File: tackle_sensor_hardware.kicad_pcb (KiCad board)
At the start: 4 copper layers, 47 x 59.7 mm, 72 parts, among them J1 Conn_ARM_JTAG_SWD_10, J2 Conn_01x02_Male, J3 Conn_01x03_Male, J4 Conn_01x04_Male, Q1 DMP4051LK3, Q2 NCE0110K, SW1 PTS645SL43SMTR92 LFS, SW2 SW_DPDT_x2, T1 DRQ125-330-R, U1 STM32G031Fx, U2 LM3488, U3 LIS2DE12, U4 LD1117S33TR_SOT223, U5 ULN2003ADR

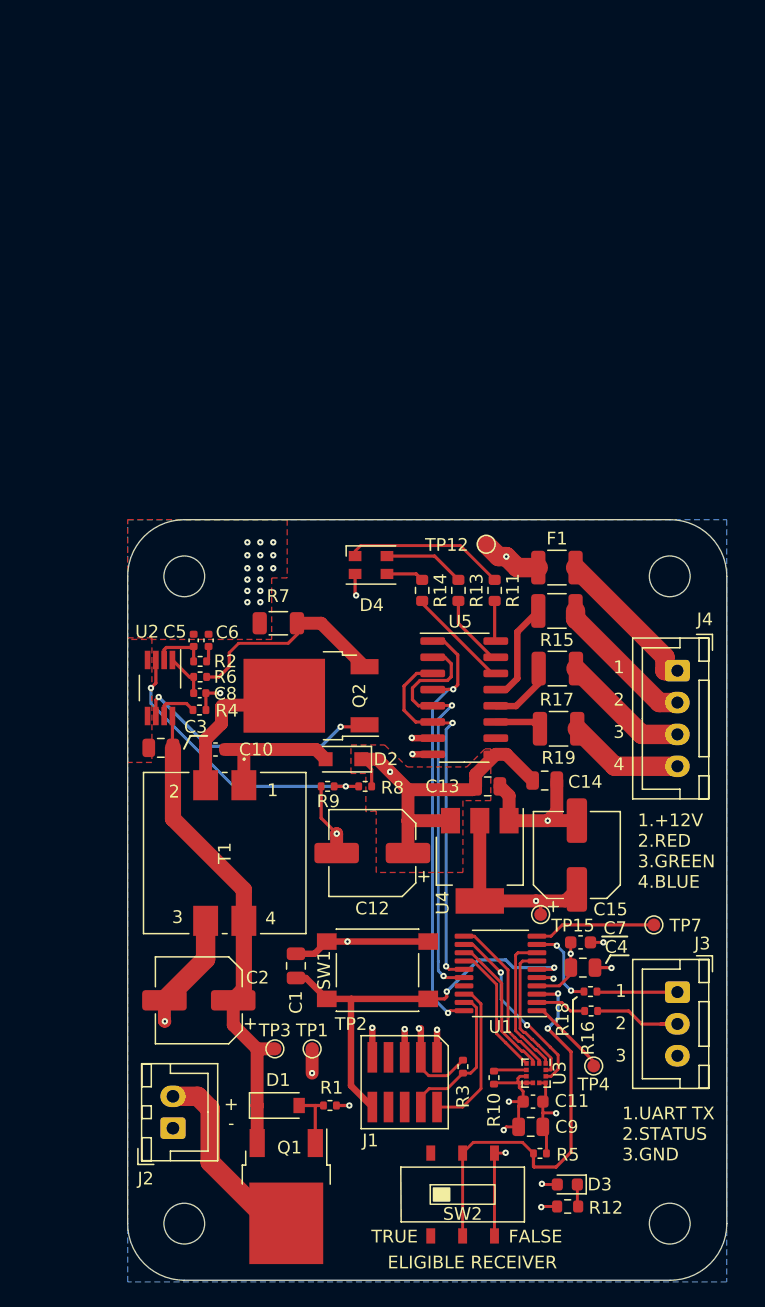
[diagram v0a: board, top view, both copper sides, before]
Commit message: - add reference PDFs and dimensions to the layout
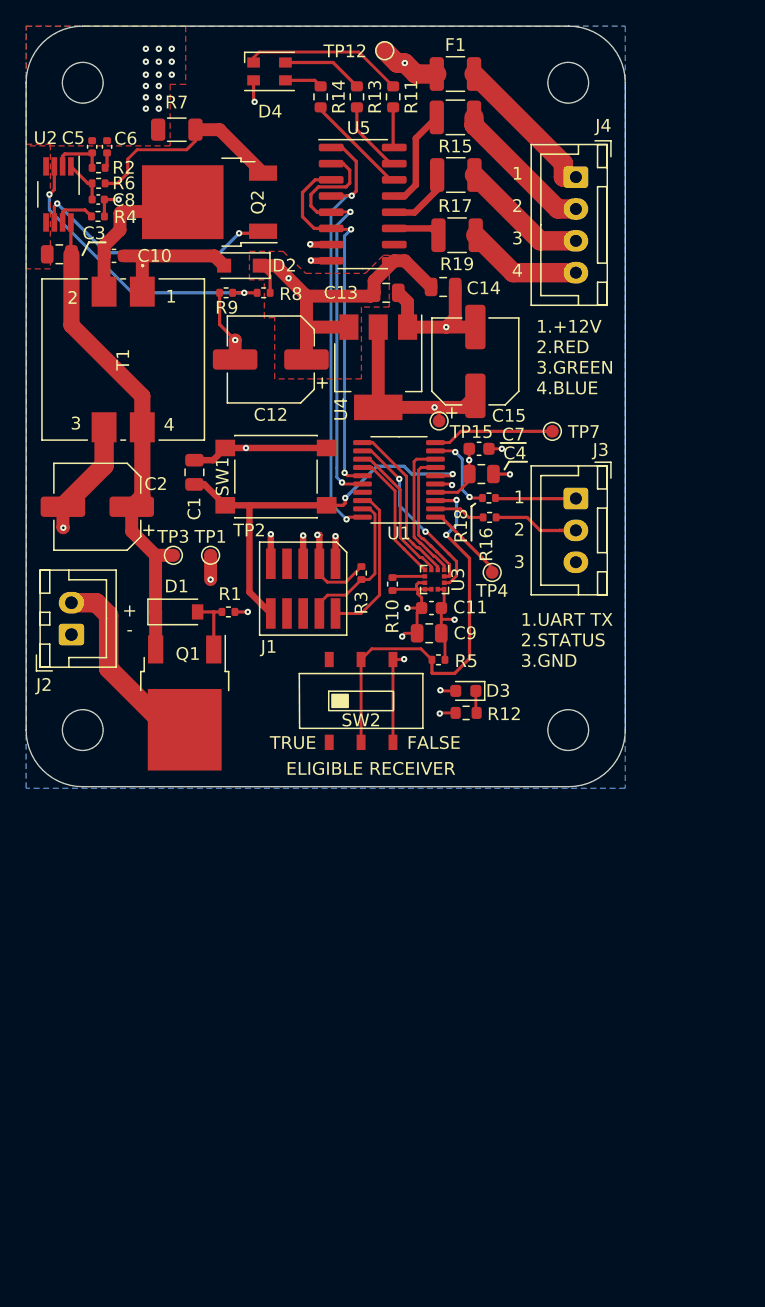
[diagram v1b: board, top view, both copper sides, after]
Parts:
- moved C14 39.5 mm to (145.4, 51.6)
- moved C15 39.5 mm to (147.9, 57.4)
- moved D1 39.5 mm to (124.5, 77.1)
- moved F1 39.5 mm to (146.4, 34.9)
- moved J1 39.5 mm to (134.4, 75.3)
- moved R10 39.5 mm to (141.4, 74.9)
- moved R12 39.5 mm to (147.2, 85.0)
- moved R14 39.5 mm to (135.8, 36.7)
- moved R15 39.5 mm to (146.4, 38.3)
- moved R3 39.5 mm to (139.0, 74.0)
- moved R5 39.5 mm to (145.0, 80.8)
- moved R9 39.5 mm to (128.4, 52.0)
- moved SW1 39.5 mm to (132.3, 66.5)
- moved TP12 39.5 mm to (140.8, 33.0)
- moved TP13 39.5 mm to (144.4, 71.9)
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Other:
- board text added: "Electrical Connector Details Power Connector - J2 Pin 1 - GND Pin 2 - V+ (10V to 30V) Status Connector - J3 (Optional) Pin 1 - UART TX (115200 bps, 8N1, 3.3V Logic Output) Pin 2 - STATUS (3.3V Logic Output) Pin 3 - GND LED Connector - J4 (Common Anode RGB LED) Pin 1 - +12V Pin 2 - RED Pin 3 - GREEN Pin 4 - BLUE"
